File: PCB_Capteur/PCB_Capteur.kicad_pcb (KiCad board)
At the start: 2 copper layers, 66 x 61 mm, 15 parts, among them J1 Conn_01x08_Socket, J2 Conn_ESP32_Custom, J3 Conn_01x02_Socket, U1 DM-OLED096-636

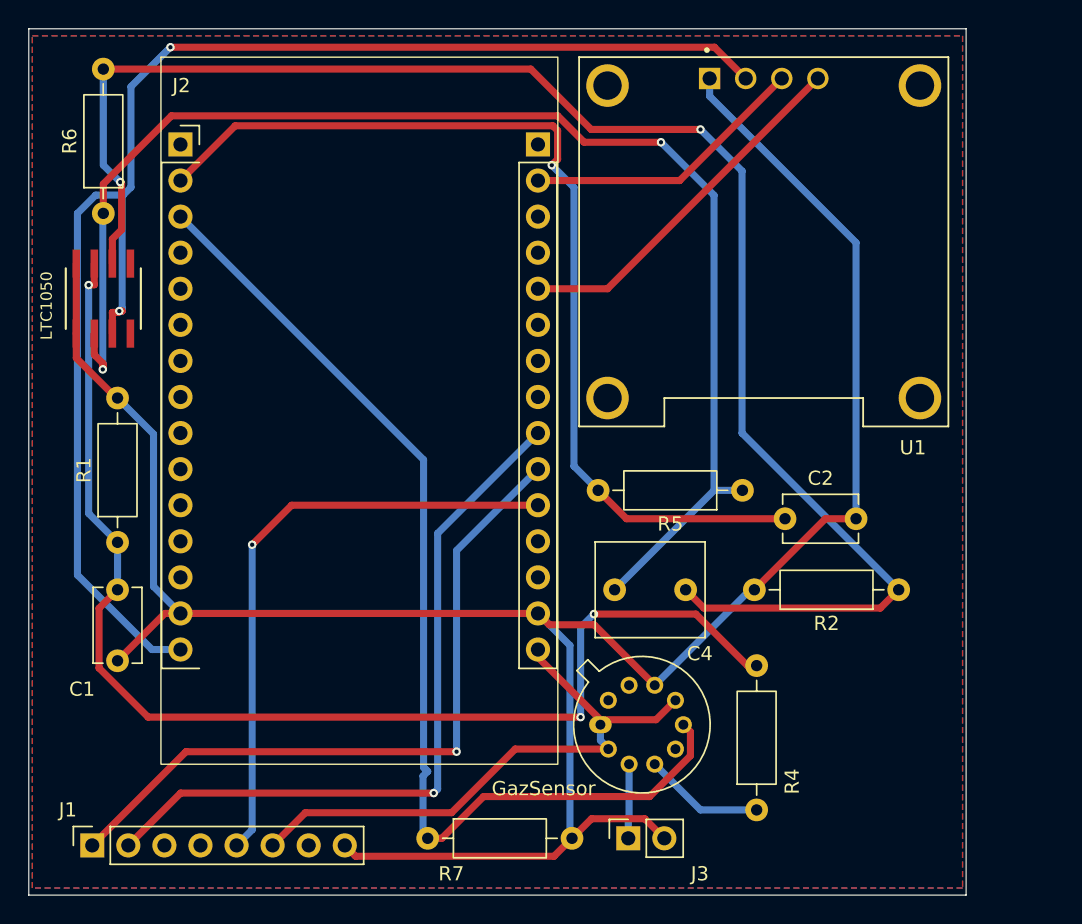
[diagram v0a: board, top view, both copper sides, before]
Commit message: PCB Improvements
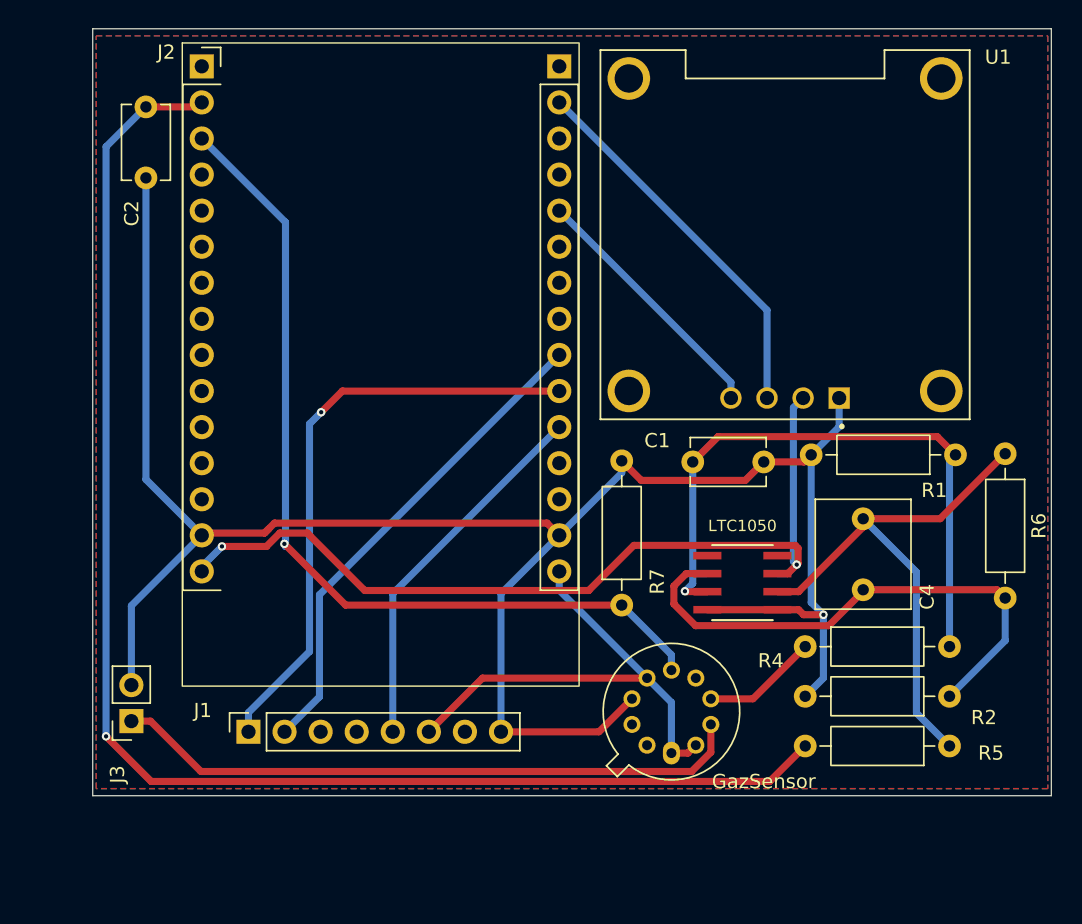
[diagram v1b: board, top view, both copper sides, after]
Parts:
- moved R6 65.7 mm to (156.5, 83.9), turned to -90 degrees
- moved R1 59.3 mm to (153.0, 84.0), turned to 180 degrees
- moved C2 53.5 mm to (96.0, 59.5), turned to -90 degrees
- moved LTC1050 49.2 mm to (138.0, 93.0), turned to 0 degrees
- moved C1 41.5 mm to (134.5, 84.5), turned to 0 degrees
- moved J3 35.9 mm to (95.0, 102.8), turned to 180 degrees
- moved R5 23.2 mm to (152.6, 104.5)
- moved R7 21.4 mm to (129.5, 94.6), turned to 90 degrees
- moved J1 13.6 mm to (103.2, 103.5)
- moved C4 12.5 mm to (146.5, 93.5), turned to 90 degrees
- moved R4 12.0 mm to (142.4, 97.5), turned to 0 degrees
- moved R2 8.31 mm to (152.6, 101.0)
- moved J2 5.70 mm to (113.5, 74.5)
- moved GazSensor 5.39 mm to (133.0, 105.0), turned to 90 degrees
- moved U1 1.58 mm to (141.0, 68.5), turned to 180 degrees
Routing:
- net Net-(LTC1050--IN): track 112.6 -> 37.8 mm, vias 2 -> 0
- net Net-(LTC1050-OUT): track 97.6 -> 38.9 mm, vias 2 -> 0
- net Net-(LTC1050-+IN): track 86.2 -> 44.4 mm, vias 3 -> 1
- net +5V: track 102.9 -> 61.3 mm
- net 15V: track 5.25 -> 44.8 mm
- net ADC: track 69.1 -> 101.1 mm
- net GND: track 164.6 -> 144.2 mm, vias 0 -> 1
- net TX: track 51.4 -> 34.5 mm, vias 1 -> 0
- net RST: track 42.9 -> 26.3 mm, vias 1 -> 0
- net TempSensor: track 75.0 -> 63.1 mm, vias 0 -> 1
- net RX: track 50.7 -> 42.0 mm
- net OLED_SDA: track 25.8 -> 18.2 mm
- net OLED_SCL: track 20.1 -> 26.9 mm
- net +3.3V: track 41.4 -> 34.9 mm
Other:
- board size 66 x 61 mm -> 67.5 x 54 mm
